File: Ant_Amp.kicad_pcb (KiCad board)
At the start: 2 copper layers, 49.1 x 23 mm, 24 parts, among them J1 Conn_Coaxial, Q1 BF981

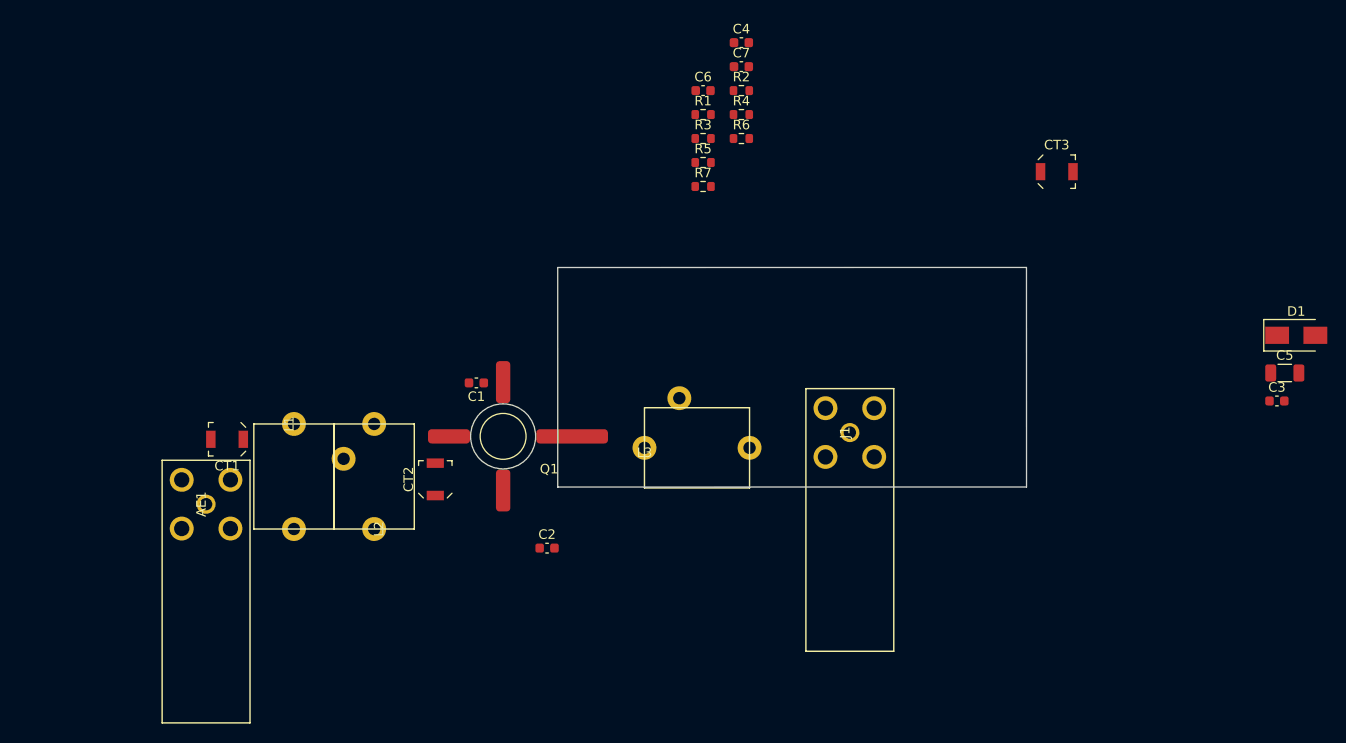
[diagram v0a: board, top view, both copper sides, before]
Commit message: 17-2-2021_02
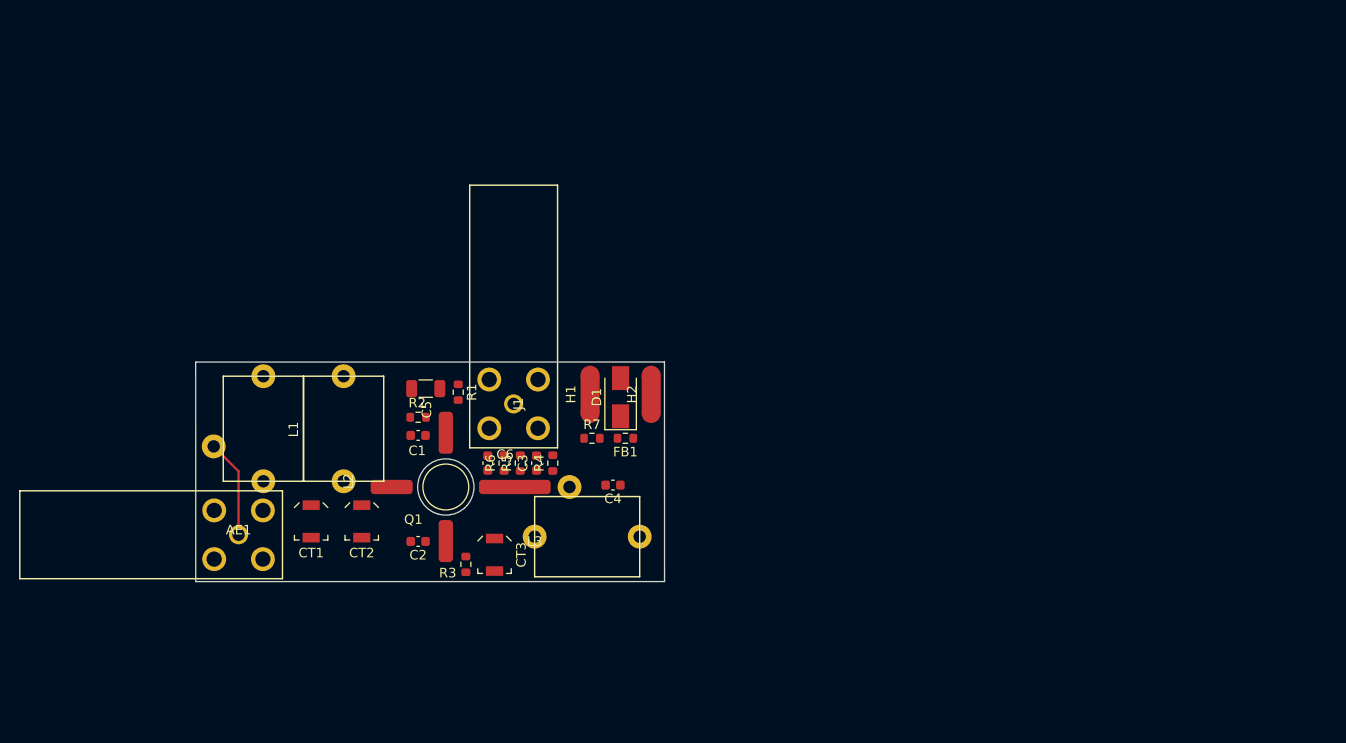
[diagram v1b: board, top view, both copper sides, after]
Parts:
- removed C7: 1nF, Capacitor_SMD:C_0603_1608Metric
- added FB1: 1k, Resistor_SMD:R_0603_1608Metric, F.Cu at (138.9, 109.4)
- added H1: MountingHole_Pad, NetTie:NetTie-2_SMD_Pad2.0mm, F.Cu at (135.2, 104.8)
- added H2: MountingHole_Pad, NetTie:NetTie-2_SMD_Pad2.0mm, F.Cu at (141.6, 104.8)
- L1: footprint Inductor:L_6T_11mm_intdiam6.3mm_1mm_wire_tap1.5T -> Inductor:L_6T_11mm_intdiam6.3mm_1mm_wire_tap1.5TL
- moved C5 90.0 mm to (118.0, 104.2), turned to 180 degrees
- moved C3 77.8 mm to (129.6, 112.0), turned to 90 degrees
- moved CT3 71.2 mm to (125.2, 121.6), turned to 270 degrees
- moved D1 71.0 mm to (138.4, 105.1), turned to 90 degrees
- moved R3 51.0 mm to (122.2, 122.6), turned to 270 degrees
- moved C4 48.2 mm to (137.6, 114.3), turned to 180 degrees
- moved R2 48.1 mm to (117.2, 107.2), turned to 180 degrees
- moved C6 45.0 mm to (124.5, 112.0), turned to 90 degrees
- moved R6 42.1 mm to (126.2, 112.0), turned to 90 degrees
- moved R4 41.5 mm to (131.3, 112.0), turned to 90 degrees
- moved R1 38.8 mm to (121.4, 104.6), turned to 270 degrees
- moved R5 36.8 mm to (127.9, 112.0), turned to 90 degrees
- moved J1 35.3 mm to (127.2, 105.8), turned to 90 degrees
- moved R7 28.8 mm to (135.4, 109.4)
- moved L3 14.8 mm to (129.4, 119.7)
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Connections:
- C5 pad 2: Net-(C5-Pad2) -> GND
- C6 pad 2: Net-(C5-Pad2) -> GND
- D1 pad 1: Net-(C4-Pad2) -> Net-(D1-Pad1)
- R7 pad 1: (no net) -> +12V
- R7 pad 2: Net-(C4-Pad2) -> Net-(D1-Pad1)
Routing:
- net Net-(AE1-Pad1): track 0.00 -> 10.3 mm

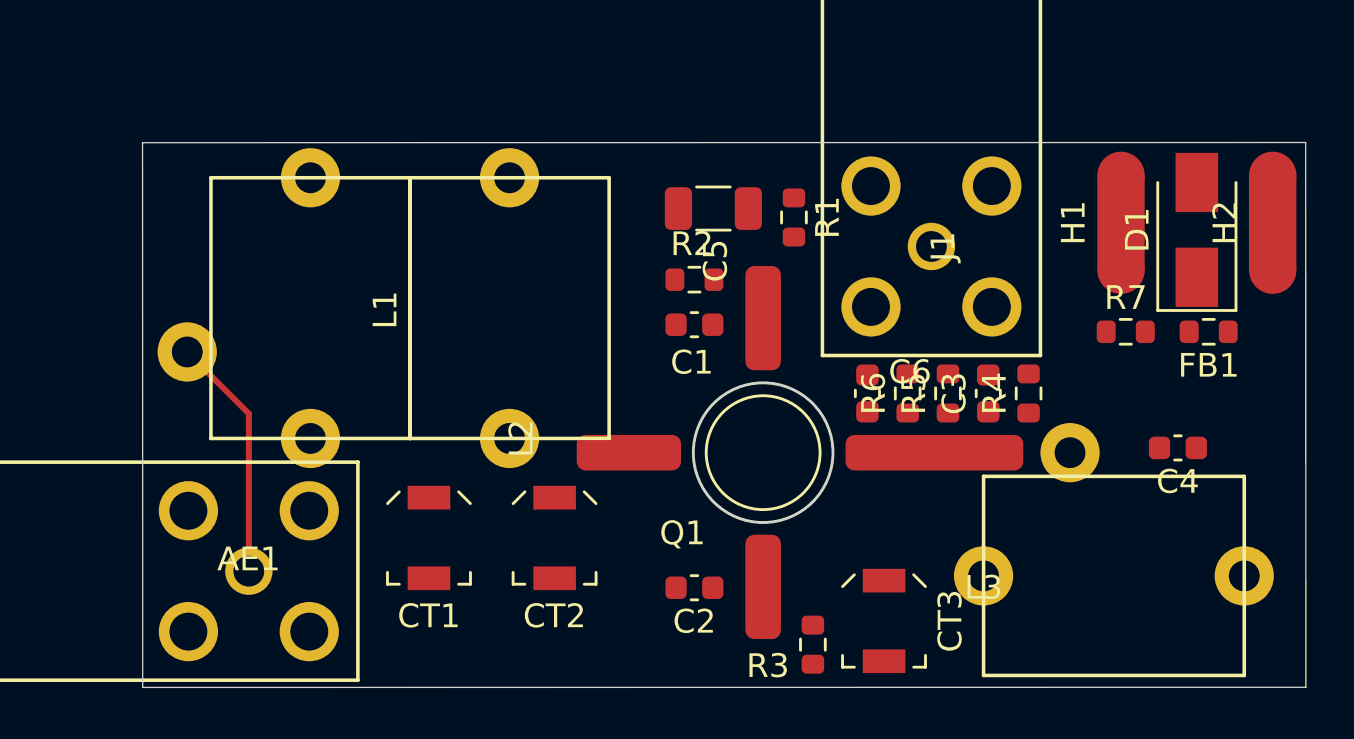
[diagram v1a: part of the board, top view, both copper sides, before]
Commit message: 17-2-21_03
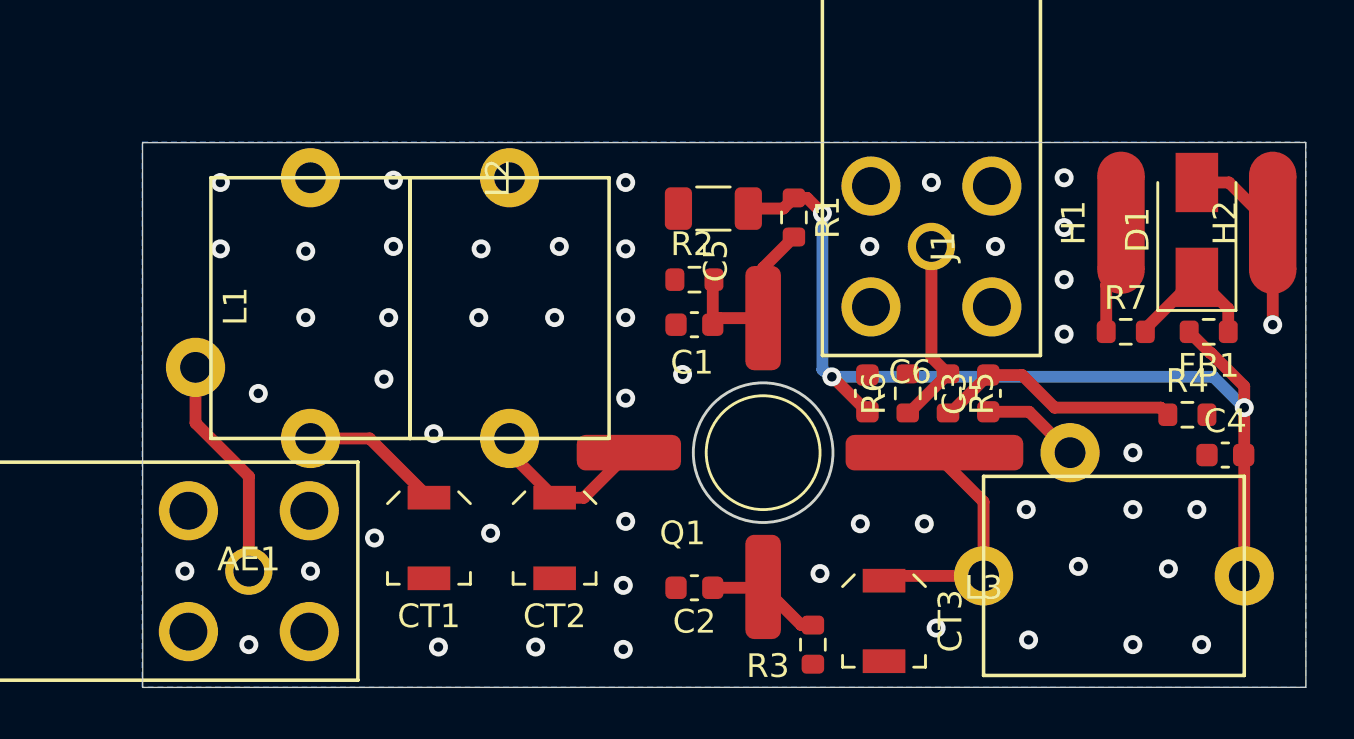
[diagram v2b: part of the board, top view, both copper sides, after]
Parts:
- H1: value MountingHole_Pad -> 12V
- H2: value MountingHole_Pad -> 0V
- L1: footprint Inductor:L_6T_11mm_intdiam6.3mm_1mm_wire_tap1.5TL -> Inductor:L_6T_11mm_intdiam6.3mm_1mm_wire_tap4.5TR
- moved L1 11.0 mm to (101.0, 102.9), turned to 270 degrees
- moved L2 11.0 mm to (109.4, 102.9), turned to 270 degrees
- moved R4 6.76 mm to (138.0, 112.9), turned to 0 degrees
- moved C4 2.02 mm to (139.6, 114.6), turned to 0 degrees
- turned R5 to 270 degrees
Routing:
- net Net-(C4-Pad2): track 0.00 -> 42.0 mm, vias 0 -> 3
- net Net-(C3-Pad2): track 0.00 -> 10.6 mm
- net Net-(CT3-Pad1): track 0.00 -> 10.3 mm
- net Net-(C1-Pad1): track 0.00 -> 8.12 mm
- net GND: track 0.00 -> 8.12 mm, vias 0 -> 50
- net Net-(J1-Pad1): track 0.00 -> 8.05 mm
- net Net-(CT2-Pad1): track 0.00 -> 7.21 mm
- net Net-(D1-Pad1): track 0.00 -> 6.05 mm
- net Net-(CT1-Pad1): track 0.00 -> 6.04 mm
- net Net-(C2-Pad1): track 0.00 -> 4.91 mm
- net Net-(C3-Pad1): track 0.00 -> 4.16 mm
- net +12V: track 0.00 -> 2.86 mm
- net Net-(AE1-Pad1): track 10.3 -> 9.53 mm
- added copper zone on B.Cu, net GND

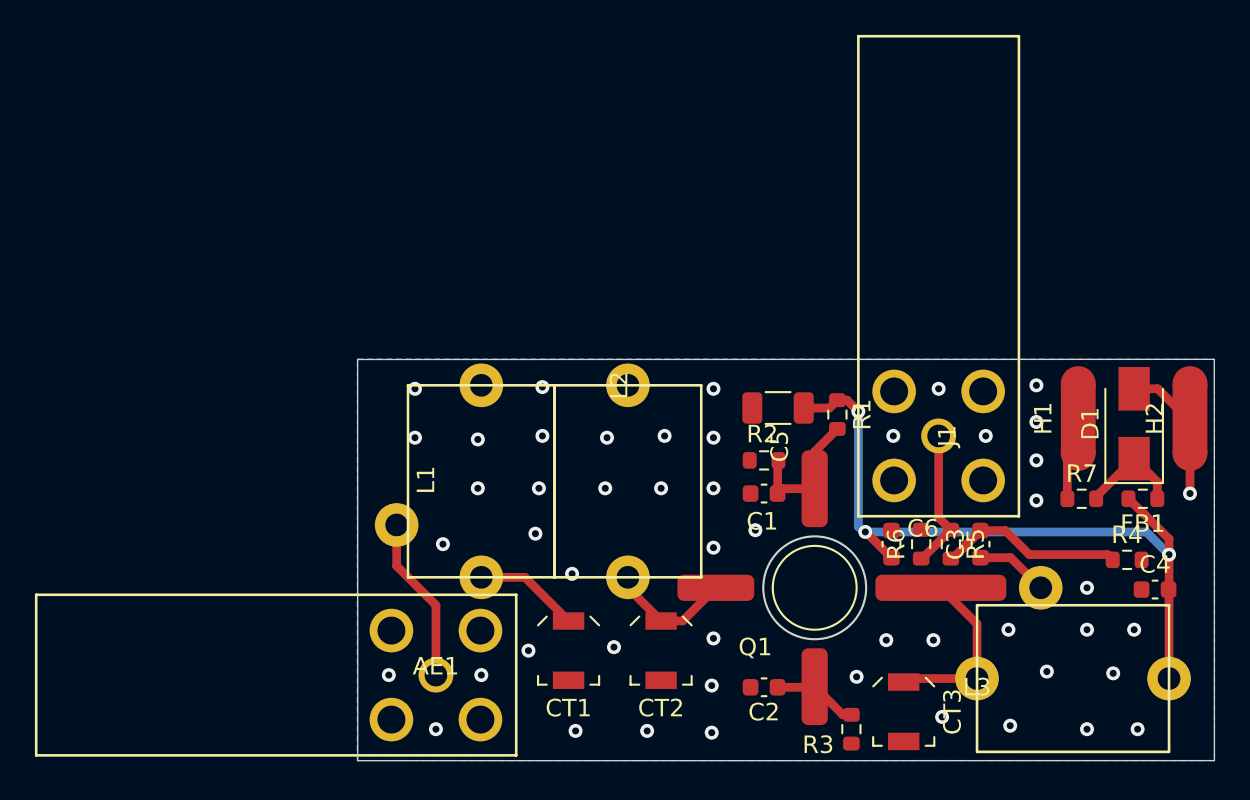
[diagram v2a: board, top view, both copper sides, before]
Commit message: Ver 1.0
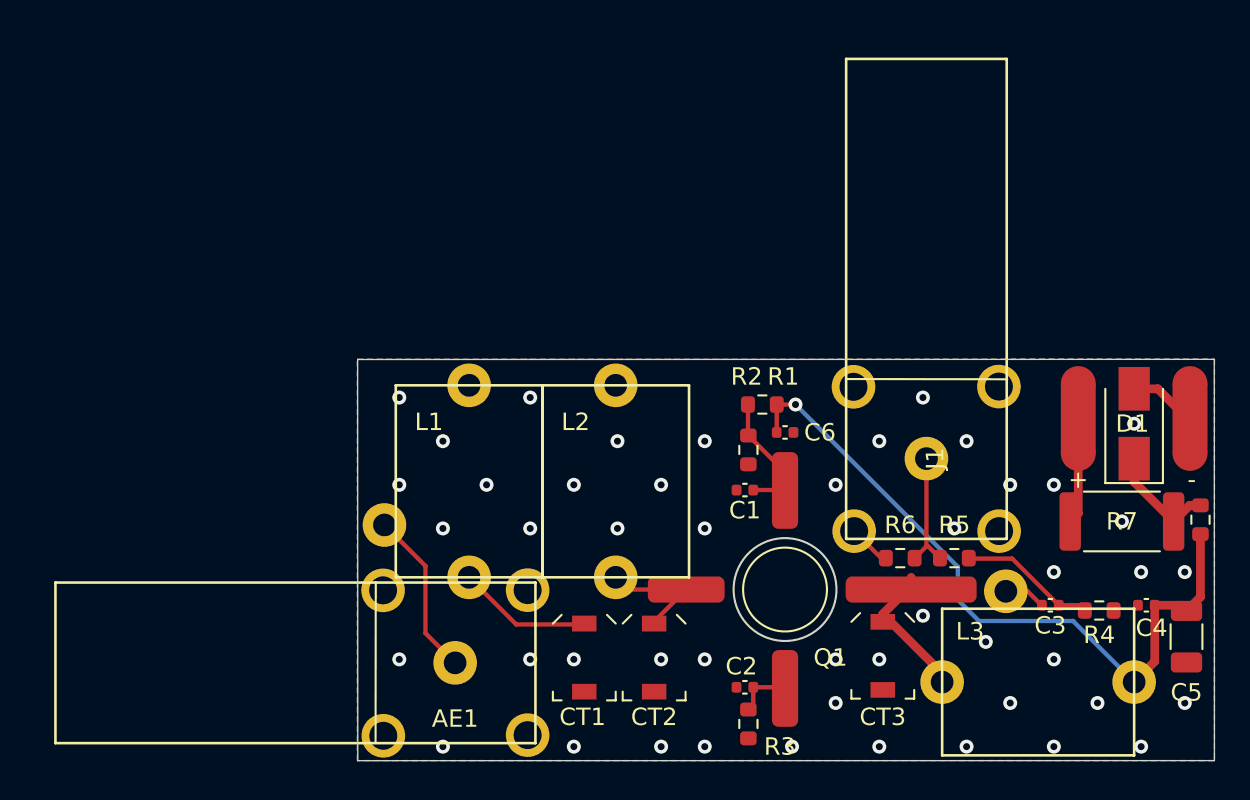
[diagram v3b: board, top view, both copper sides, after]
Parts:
- C1, C2, C3, C4, C6: footprint Capacitor_SMD:C_0603_1608Metric -> Capacitor_SMD:C_0402_1005Metric
- CT1, CT2, CT3: footprint Capacitor_SMD:C_Trimmer_Voltronics_JR -> Capacitor_SMD:C_Trimmer_Voltronics_JZ
- D1: value 10V -> SMA12JA
- R7: footprint Resistor_SMD:R_0603_1608Metric -> Resistor_SMD:R_2512_6332Metric
- moved C5 26.8 mm to (141.4, 117.3), turned to 270 degrees
- moved C6 8.84 mm to (118.4, 105.6), turned to 0 degrees
- moved R3 5.91 mm to (116.3, 122.3)
- moved C3 5.32 mm to (133.6, 115.5), turned to 180 degrees
- moved R1 4.34 mm to (117.1, 104.0), turned to 0 degrees
- moved FB1 3.51 mm to (142.2, 110.6), turned to 270 degrees
- moved CT3 3.42 mm to (124.0, 118.4)
- moved R4 3.31 mm to (136.4, 115.8)
- moved R7 2.64 mm to (137.7, 110.7)
- moved L3 2.01 mm to (127.4, 119.9)
- moved Q1 1.70 mm to (118.4, 114.6)
- moved J1 1.48 mm to (126.5, 107.1)
- moved R6 1.44 mm to (125.0, 112.8), turned to 180 degrees
- moved AE1 1.30 mm to (99.5, 118.8)
- moved C1 1.12 mm to (116.1, 108.9)
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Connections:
- L3 pad 3: Net-(C3-Pad1) -> Net-(C3-Pad2)
- R1 pad 1: Net-(C4-Pad2) -> Net-(C1-Pad1)
- R1 pad 2: Net-(C1-Pad1) -> Net-(C4-Pad2)
- R4 pad 1: Net-(C3-Pad2) -> Net-(C3-Pad1)
- R5 pad 2: Net-(C3-Pad2) -> Net-(C3-Pad1)
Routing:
- net Net-(C3-Pad2): track 10.6 -> 2.40 mm
- net Net-(C3-Pad1): track 4.16 -> 7.90 mm
- net Net-(CT3-Pad1): track 10.3 -> 7.58 mm
- net Net-(CT1-Pad1): track 6.04 -> 7.72 mm
- net Net-(C2-Pad1): track 4.91 -> 3.27 mm
- net +12V: track 2.86 -> 4.09 mm
- net Net-(J1-Pad1): track 8.05 -> 7.03 mm
- net Net-(C4-Pad2): track 42.0 -> 41.4 mm, vias 3 -> 1
- net GND: track 8.12 -> 8.27 mm, vias 50 -> 48
- added copper zone on F.Cu, net GND
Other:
- board text added: "+"
- board text added: "-"
